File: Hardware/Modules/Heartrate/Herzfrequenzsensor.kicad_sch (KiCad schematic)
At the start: 8 parts, among them U1 MAX30101EFD_T, U2 TLV70018_SOT23-5, U4 PCA9306DCTR

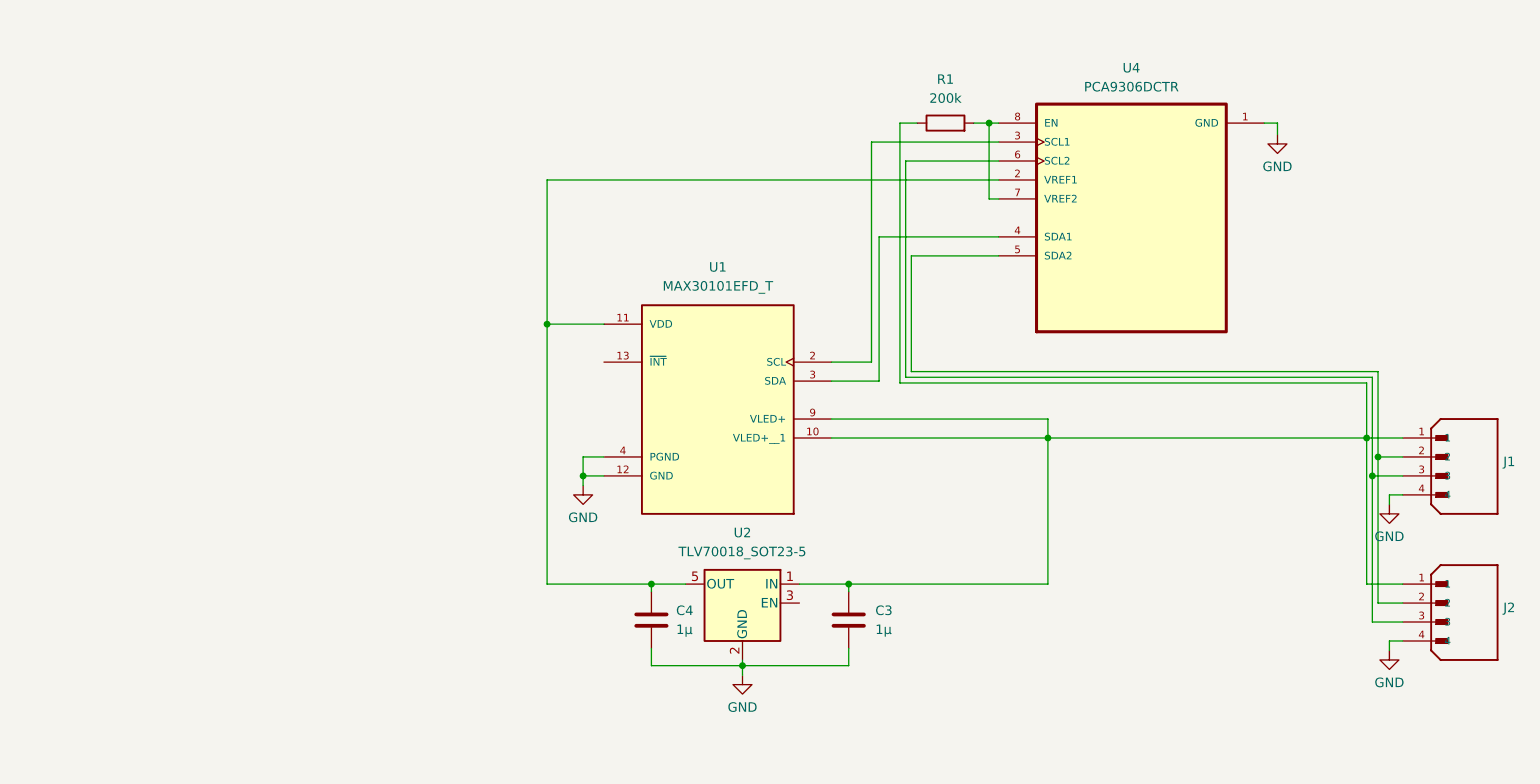
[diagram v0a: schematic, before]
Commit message: HeartRateV2
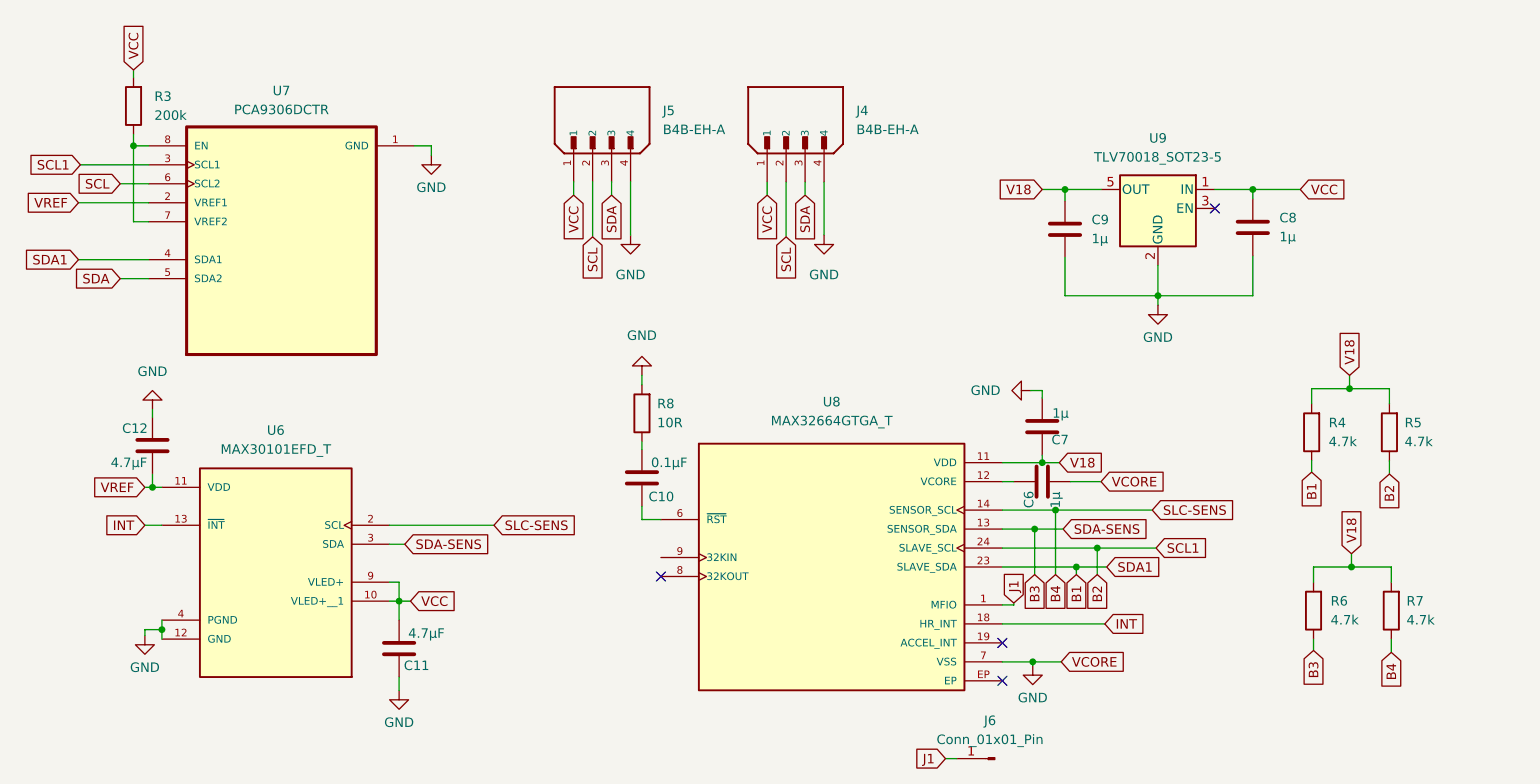
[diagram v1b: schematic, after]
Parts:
- removed C3, C4: 1µ, Capacitor_SMD:C_0603_1608Metric_Pad1.08x0.95mm_HandSolder, symbol Device:C
- removed J1, J2: ~, Connector_JST:JST_EH_B4B-EH-A_1x04_P2.50mm_Vertical, symbol Modular_Electronics_Toolkit:CONN_I2C
- removed R1: 200k, Resistor_SMD:R_0603_1608Metric_Pad0.98x0.95mm_HandSolder, symbol Device:R
- removed U1: MAX30101EFD_T, Modular_Electronics_Toolkit:PSON80P560X330X165-14N, symbol Modular_Electronics_Toolkit:MAX30101EFD_T
- removed U2: TLV70018_SOT23-5, Package_TO_SOT_SMD:SOT-23-5, symbol Regulator_Linear:TLV70018_SOT23-5
- removed U4: PCA9306DCTR, Modular_Electronics_Toolkit:SOP65P400X130-8N, symbol Modular_Electronics_Toolkit:PCA9306DCTR
- added C10: 0.1µF, Capacitor_SMD:C_0603_1608Metric_Pad1.08x0.95mm_HandSolder, symbol Device:C
- added C11, C12: 4.7µF, Capacitor_SMD:C_0603_1608Metric_Pad1.08x0.95mm_HandSolder, symbol Device:C
- added C6, C7, C8, C9: 1µ, Capacitor_SMD:C_0603_1608Metric_Pad1.08x0.95mm_HandSolder, symbol Device:C
- added J4, J5: B4B-EH-A, Connector_JST:JST_EH_B4B-EH-A_1x04_P2.50mm_Vertical, symbol Modular_Electronics_Toolkit_sym:B4B-EH-A
- added J6: Conn_01x01_Pin, Connector_PinHeader_2.54mm:PinHeader_1x01_P2.54mm_Vertical, symbol Connector:Conn_01x01_Pin
- added R3: 200k, Resistor_SMD:R_0603_1608Metric_Pad0.98x0.95mm_HandSolder, symbol Device:R
- added R4, R5, R6, R7: 4.7k, Resistor_SMD:R_0603_1608Metric_Pad0.98x0.95mm_HandSolder, symbol Device:R
- added R8: 10R, Resistor_SMD:R_0603_1608Metric_Pad0.98x0.95mm_HandSolder, symbol Device:R
- added U6: MAX30101EFD_T, Modular_Electronics_Toolkit:PSON80P560X330X165-14N, symbol Modular_Electronics_Toolkit:MAX30101EFD_T
- added U7: PCA9306DCTR, Modular_Electronics_Toolkit:SOP65P400X130-8N, symbol Modular_Electronics_Toolkit:PCA9306DCTR
- added U8: MAX32664GTGA_T, Modular_Electronics_Toolkit:IC_MAX32664GTGA_T, symbol Modular_Electronics_Toolkit_sym:MAX32664GTGA_T
- added U9: TLV70018_SOT23-5, Package_TO_SOT_SMD:SOT-23-5, symbol Regulator_Linear:TLV70018_SOT23-5
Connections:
- net GND: now also C11.2, C12.2, C6.1, C7.1, C8.2, C9.2, J4.4, J5.4, R8.2, U6.12 (GND), U6.4 (PGND), U7.1 (GND), U8.10 (VSS__1), U8.7 (VSS), U9.2 (GND)
- new net: C6.2, U8.12 (VCORE)
- new net: C10.1, R8.1
- new net: R3.1, U7.7 (VREF2), U7.8 (EN)
- new net: C10.2, U8.6 (~{RST})
- new net B1: R4.1, U7.4 (SDA1), U8.23 (SLAVE_SDA)
- new net B2: R5.1, U7.3 (SCL1), U8.24 (SLAVE_SCL)
- new net B3: R6.1, U6.3 (SDA), U8.13 (SENSOR_SDA)
- new net B4: R7.1, U6.2 (SCL), U8.14 (SENSOR_SCL)
- new net INT: U6.13 (~{INT}), U8.18 (HR_INT)
- new net J1: J6.1 (Pin_1), U8.1 (MFIO)
- new net SCL: J4.2, J5.2, U7.6 (SCL2)
- new net SDA: J4.3, J5.3, U7.5 (SDA2)
- new net VCC: C11.1, C8.1, J4.1, J5.1, R3.2, U6.10 (VLED+__1), U6.9 (VLED+), U9.1 (IN)
- new net VDD__1: C7.2, C9.1, R4.2, R5.2, R6.2, R7.2, U8.11 (VDD), U8.22 (VDD__1), U9.5 (OUT)
- new net VREF: C12.1, U6.11 (VDD), U7.2 (VREF1)
- no-connect marks 0 -> 4
